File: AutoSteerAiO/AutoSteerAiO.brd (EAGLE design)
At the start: 114.3 x 99.1 mm, 87 parts, among them J4 CONNECTOR 1x5 PINS, K4 CB1A-P-12V, T1 BC547, U1 VX7805-1000

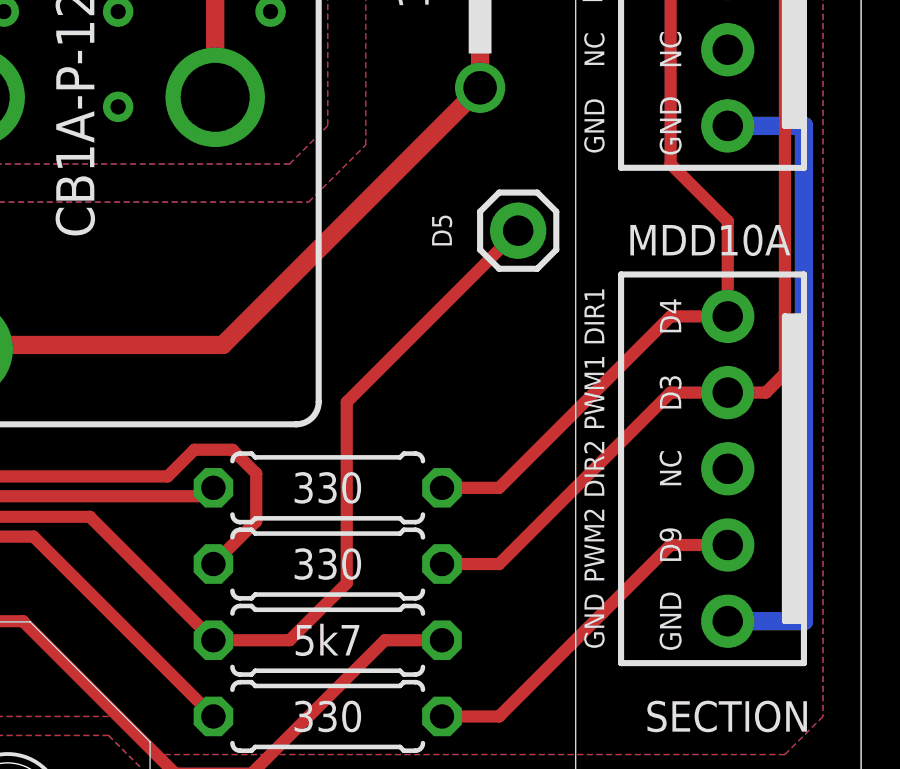
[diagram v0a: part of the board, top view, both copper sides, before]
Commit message: Add files via upload
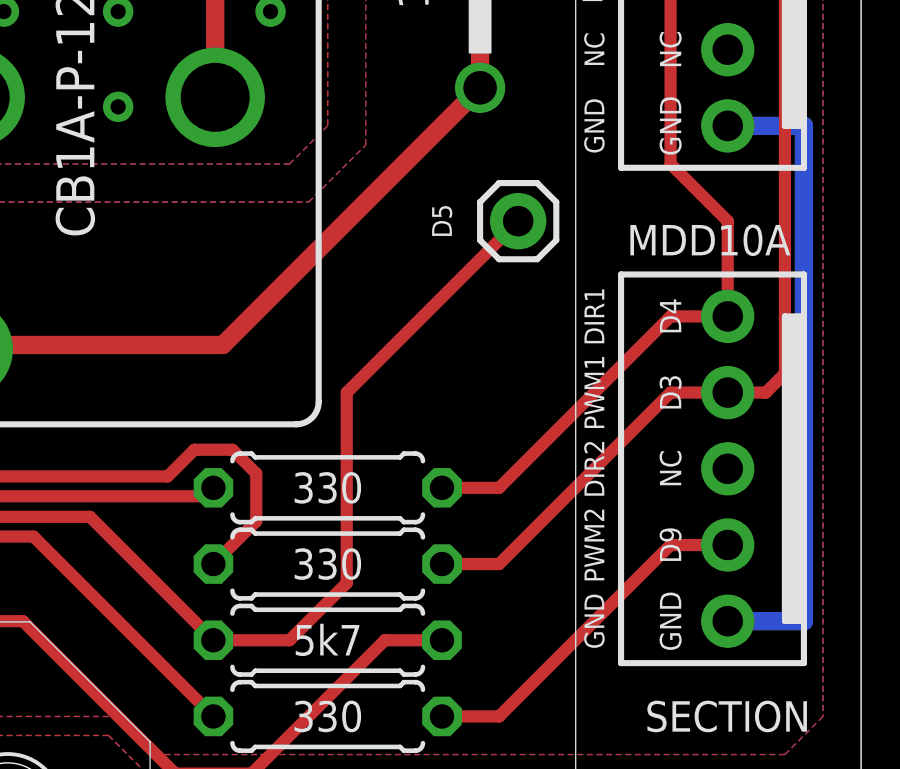
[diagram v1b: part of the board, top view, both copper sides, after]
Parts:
- moved D5 0.32 mm to (102.9, 62.9)
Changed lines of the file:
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@@
 <attribute name="OC_NEWARK" value="unknown" x="43.18" y="24.13" size="1.778" layer="27" display="off"/>
 </element>
-<element name="D5" library="SparkFun-Connectors" library_urn="urn:adsk.eagle:library:513" package="1X01" package3d_urn="urn:adsk.eagle:package:38028/1" value="CONNECTOR 1x1 PIN" x="102.87" y="62.5475" smashed="yes" rot="R90">
-<attribute name="MF" value="" x="102.87" y="62.5475" size="1.778" layer="27" rot="R90" display="off"/>
-<attribute name="MPN" value="" x="102.87" y="62.5475" size="1.778" layer="27" rot="R90" display="off"/>
-<attribute name="NAME" x="100.33" y="62.5475" size="0.6604" layer="25" font="vector" ratio="15" rot="R270" align="center"/>
-<attribute name="OC_NEWARK" value="unknown" x="102.87" y="62.5475" size="1.778" layer="27" rot="R90" display="off"/>
+<element name="D5" library="SparkFun-Connectors" library_urn="urn:adsk.eagle:library:513" package="1X01" package3d_urn="urn:adsk.eagle:package:38028/1" value="CONNECTOR 1x1 PIN" x="102.87" y="62.865" smashed="yes" rot="R90">
+<attribute name="MF" value="" x="102.87" y="62.865" size="1.778" layer="27" rot="R90" display="off"/>
+<attribute name="MPN" value="" x="102.87" y="62.865" size="1.778" layer="27" rot="R90" display="off"/>
+<attribute name="NAME" x="100.33" y="62.865" size="0.6604" layer="25" font="vector" ratio="15" rot="R270" align="center"/>
+<attribute name="OC_NEWARK" value="unknown" x="102.87" y="62.865" size="1.778" layer="27" rot="R90" display="off"/>
 </element>
 <element name="0" library="SparkFun-Connectors" library_urn="urn:adsk.eagle:library:513" package="1X03" package3d_urn="urn:adsk.eagle:package:38063/1" value="CONNECTOR 1x2 PINS" x="61.595" y="4.445" smashed="yes">
@@
 <wire x1="88.5952" y1="53.0098" x2="92.71" y2="48.895" width="0.4064" layer="1"/>
 <contactref element="D5" pad="1"/>
-<wire x1="102.87" y1="62.5475" x2="97.155" y2="56.8325" width="0.4064" layer="1"/>
-<wire x1="97.155" y1="56.8325" x2="97.155" y2="50.8" width="0.4064" layer="1"/>
+<wire x1="102.87" y1="62.865" x2="97.155" y2="57.15" width="0.4064" layer="1"/>
+<wire x1="97.155" y1="57.15" x2="97.155" y2="50.8" width="0.4064" layer="1"/>
 <wire x1="92.71" y1="48.895" x2="95.25" y2="48.895" width="0.4064" layer="1"/>
 <wire x1="95.25" y1="48.895" x2="97.155" y2="50.8" width="0.4064" layer="1"/>
